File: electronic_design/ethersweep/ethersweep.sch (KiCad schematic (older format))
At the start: 98 parts, among them J1 AVR-ISP-6, J10 HR911105A, J11 B4B-XH-A(LF)(SN), J2 Conn_01x02_Male, J3 Conn_01x04_Female, J4 Conn_01x02_Male, J5 Conn_01x02_Male, J6 Conn_01x07_Female, J7 Conn_01x07_Male, J8 AVR-ISP-6, J9 USB_B_Micro, M1 Stepper_Motor_bipolar, SW1 SW_Push, U1 CP2102N-A01-GQFN28, U2 ATmega328-AU, U3 TMC2208-LA-T, U4 DD4012SA, U5 AS5600, U6 W5500, Y2 Crystal_25MHz, Y3 Crystal

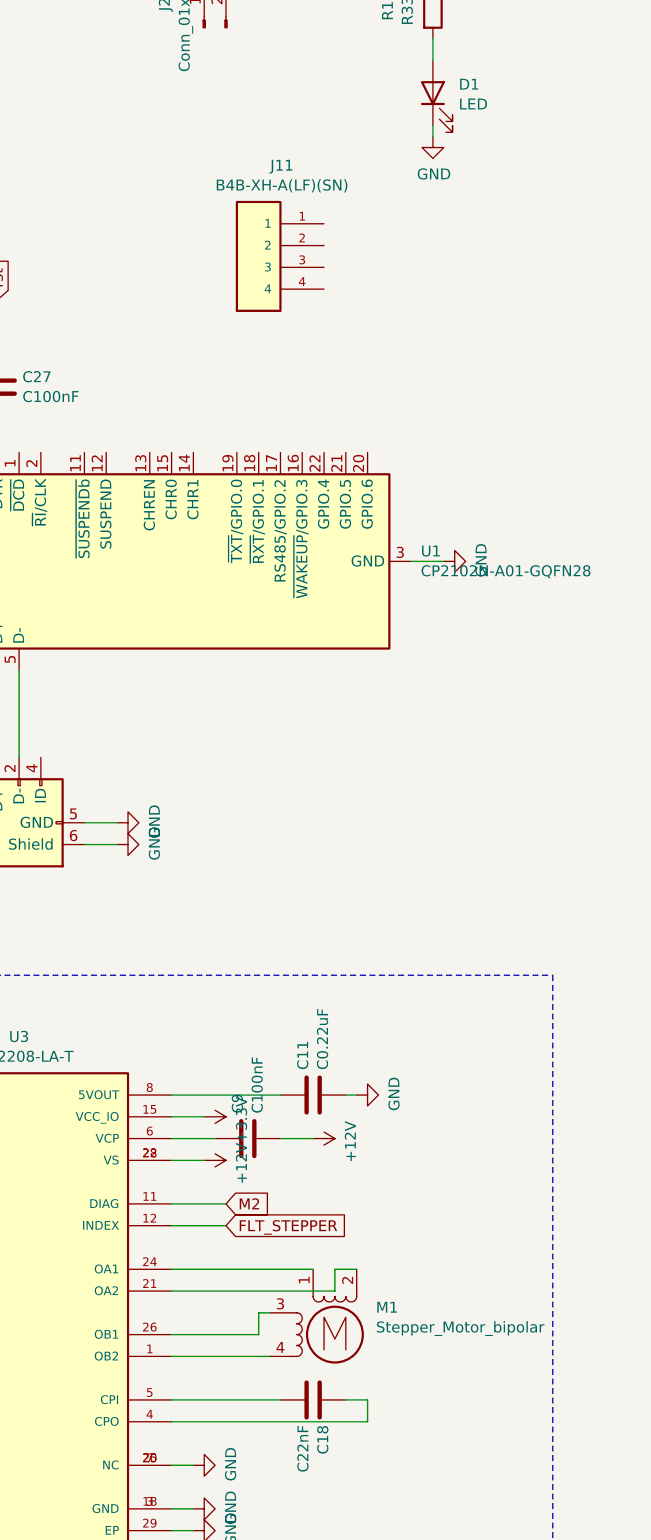
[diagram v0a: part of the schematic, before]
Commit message: added 3d cad files, production files, for 3.0.4
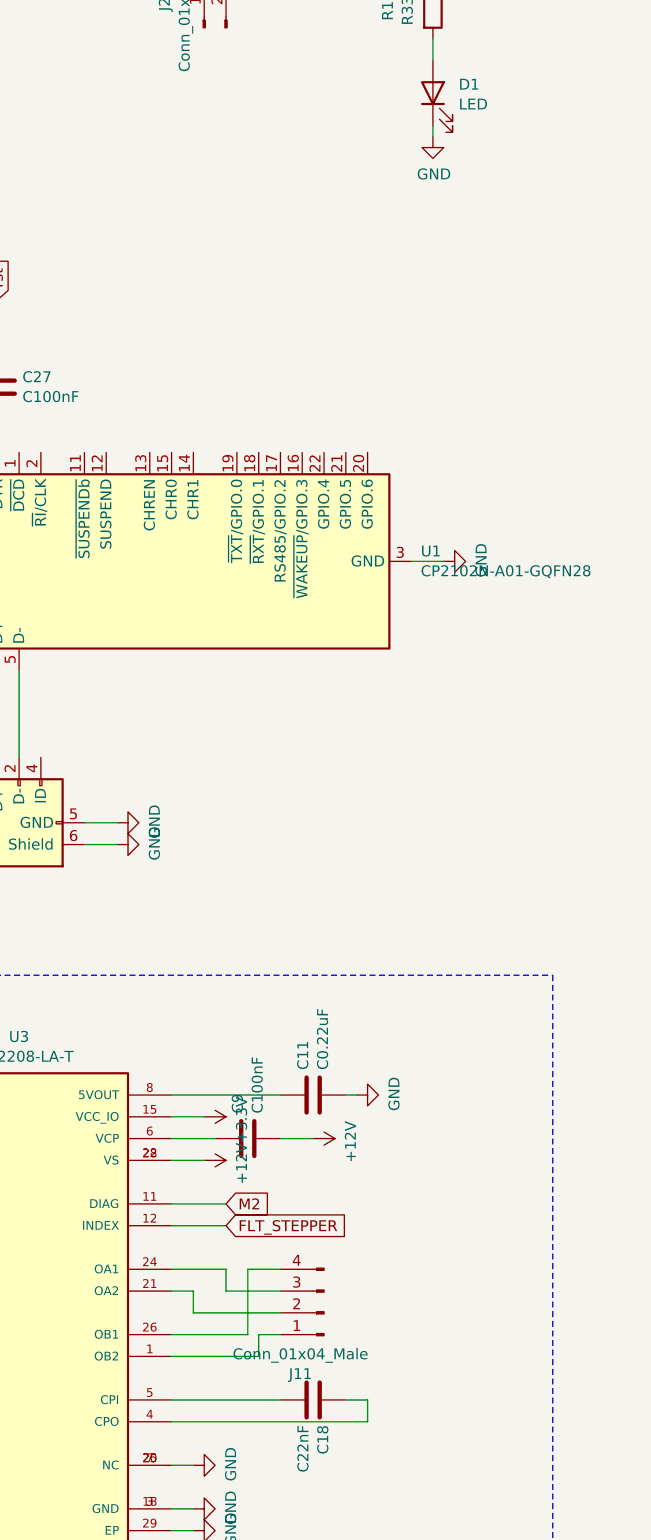
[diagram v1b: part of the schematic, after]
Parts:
- removed J11: B4B-XH-A(LF)(SN), modules:JST_B4B-XH-A(LF)(SN), symbol B4B-XH-A_LF__SN_:B4B-XH-A(LF)(SN)
- removed M1: Stepper_Motor_bipolar, Connector_PinHeader_2.54mm:PinHeader_2x02_P2.54mm_Vertical_SMD, symbol Motor:Stepper_Motor_bipolar
- added J11: Conn_01x04_Male, Connector_JST:JST_EH_S4B-EH_1x04_P2.50mm_Horizontal, symbol Connector:Conn_01x04_Male
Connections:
- net at U3.1 (OB2): now also J11.1 (Pin_1)
- net at U3.21 (OA2): now also J11.2 (Pin_2)
- net at U3.24 (OA1): now also J11.3 (Pin_3)
- net at U3.26 (OB1): now also J11.4 (Pin_4)
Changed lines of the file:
@@
 	12600 6900 12350 6900
-$Comp
-L Motor:Stepper_Motor_bipolar M1
-U 1 1 611E7EF6
-P 14750 7400
-F 0 "M1" H 14938 7524 50  0000 L CNN
-F 1 "Stepper_Motor_bipolar" H 14938 7433 50  0000 L CNN
-F 2 "Connector_PinHeader_2.54mm:PinHeader_2x02_P2.54mm_Vertical_SMD" H 14760 7390 50  0001 C CNN
-F 3 "http://www.infineon.com/dgdl/Application-Note-TLE8110EE_driving_UniPolarStepperMotor_V1.1.pdf?fileId=db3a30431be39b97011be5d0aa0a00b0" H 14760 7390 50  0001 C CNN
-	1    14750 7400
-	1    0    0    -1
-$EndComp
-Wire Wire Line
-	14400 7400 14400 7300
-Wire Wire Line
-	14400 7300 14450 7300
-Wire Wire Line
-	14750 7100 14850 7100
 $Comp
 L Device:C C18
@@
 Wire Wire Line
 	14000 8200 14100 8200
-Wire Wire Line
-	14000 7100 14650 7100
-Wire Wire Line
-	14000 7200 14750 7200
-Wire Wire Line
-	14750 7100 14750 7200
-Wire Wire Line
-	14000 7400 14400 7400
-Wire Wire Line
-	14000 7500 14450 7500
 $Comp
 L Device:R R12
@@
 Wire Wire Line
 	12400 4500 13000 4500
-$Comp
-L B4B-XH-A_LF__SN_:B4B-XH-A(LF)(SN) J11
-U 1 1 622C08A7
-P 14400 2500
-F 0 "J11" H 14507 2967 50  0000 C CNN
-F 1 "B4B-XH-A(LF)(SN)" H 14507 2876 50  0000 C CNN
-F 2 "modules:JST_B4B-XH-A(LF)(SN)" H 14400 2500 50  0001 L BNN
-F 3 "" H 14400 2500 50  0001 L BNN
-F 4 "Manufacturer Recommendation" H 14400 2500 50  0001 L BNN "STANDARD"
-F 5 "NA" H 14400 2500 50  0001 L BNN "PARTREV"
-F 6 "JST Sales America Inc" H 14400 2500 50  0001 L BNN "MANUFACTURER"
-	1    14400 2500
-	1    0    0    -1
-$EndComp
 Wire Notes Line
 	15750 9650 11250 9650
@@
 	0    -1   -1   0
 $EndComp
+$Comp
+L Connector:Conn_01x04_Male J11
+U 1 1 61920619
+P 14700 7300
+F 0 "J11" H 14808 7581 50  0000 C CNN
+F 1 "Conn_01x04_Male" H 14808 7490 50  0000 C CNN
+F 2 "Connector_JST:JST_EH_S4B-EH_1x04_P2.50mm_Horizontal" H 14700 7300 50  0001 C CNN
+F 3 "~" H 14700 7300 50  0001 C CNN
+	1    14700 7300
+	-1   0    0    1
+$EndComp
+Wire Wire Line
+	14000 7100 14250 7100
+Wire Wire Line
+	14250 7100 14250 7200
+Wire Wire Line
+	14250 7200 14500 7200
+Wire Wire Line
+	14350 7100 14350 7400
+Wire Wire Line
+	14350 7400 14000 7400
+Wire Wire Line
+	14350 7100 14500 7100
+Wire Wire Line
+	14000 7200 14100 7200
+Wire Wire Line
+	14100 7200 14100 7300
+Wire Wire Line
+	14100 7300 14500 7300
+Wire Wire Line
+	14500 7400 14400 7400
+Wire Wire Line
+	14400 7400 14400 7500
+Wire Wire Line
+	14400 7500 14000 7500
 $EndSCHEMATC

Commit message: removed old code + design files
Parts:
- RV1: footprint Potentiometer_THT:Potentiometer_Bourns_3296W_Vertical -> Potentiometer_SMD:Potentiometer_Bourns_TC33X_Vertical; LCSC (none) -> C719177
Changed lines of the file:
@@
 F 0 "RV1" H 12130 6096 50  0000 R CNN
 F 1 "R_POT_20K" H 12130 6005 50  0000 R CNN
-F 2 "Potentiometer_THT:Potentiometer_Bourns_3296W_Vertical" H 12200 6050 50  0001 C CNN
+F 2 "Potentiometer_SMD:Potentiometer_Bourns_TC33X_Vertical" H 12200 6050 50  0001 C CNN
 F 3 "~" H 12200 6050 50  0001 C CNN
-F 4 "" H 12200 6050 50  0001 C CNN "LCSC"
+F 4 "C719177" H 12200 6050 50  0001 C CNN "LCSC"
 	1    12200 6050
 	0    1    1    0
